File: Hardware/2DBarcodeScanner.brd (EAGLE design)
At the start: 43.2 x 35.6 mm, 53 parts, among them J1 BARCODE_ENGINE_CONN, Q1 600mA/40V, Q2 600mA/40V, U1 3.3V, U5 CH340C

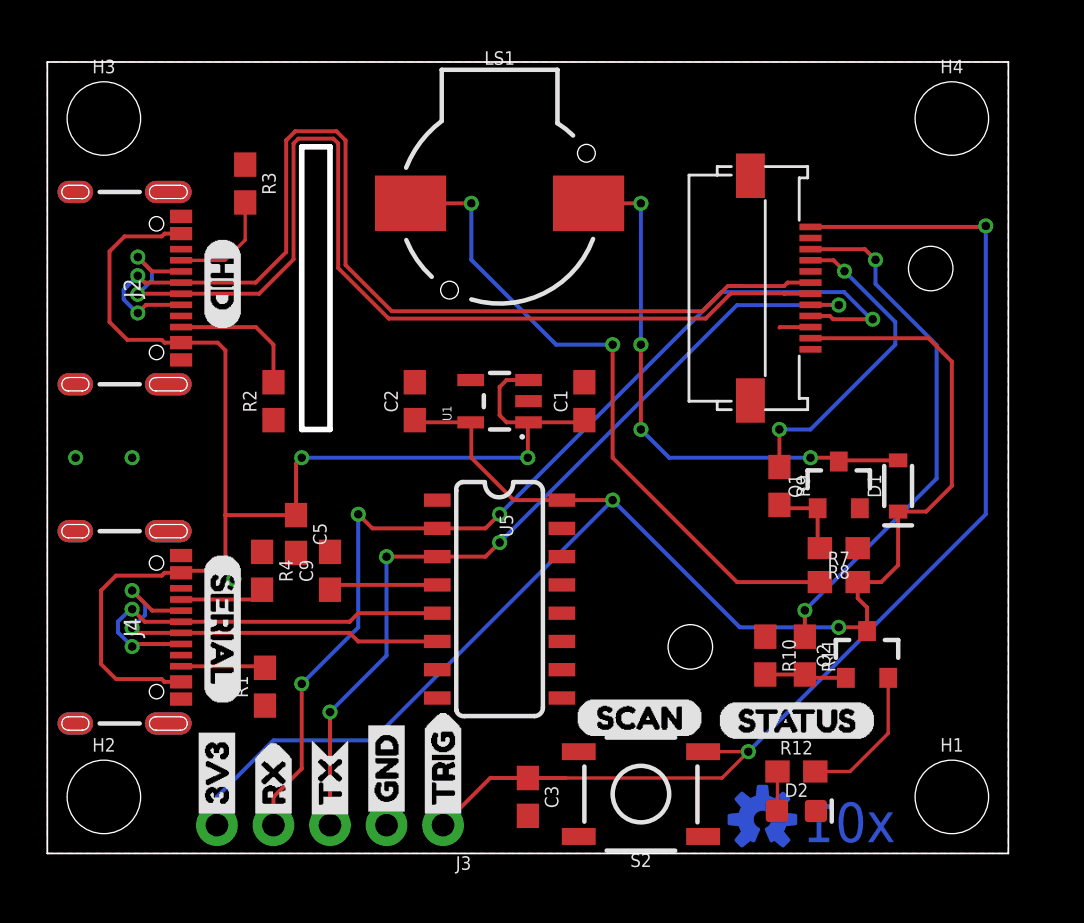
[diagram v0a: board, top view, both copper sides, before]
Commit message: Version x02
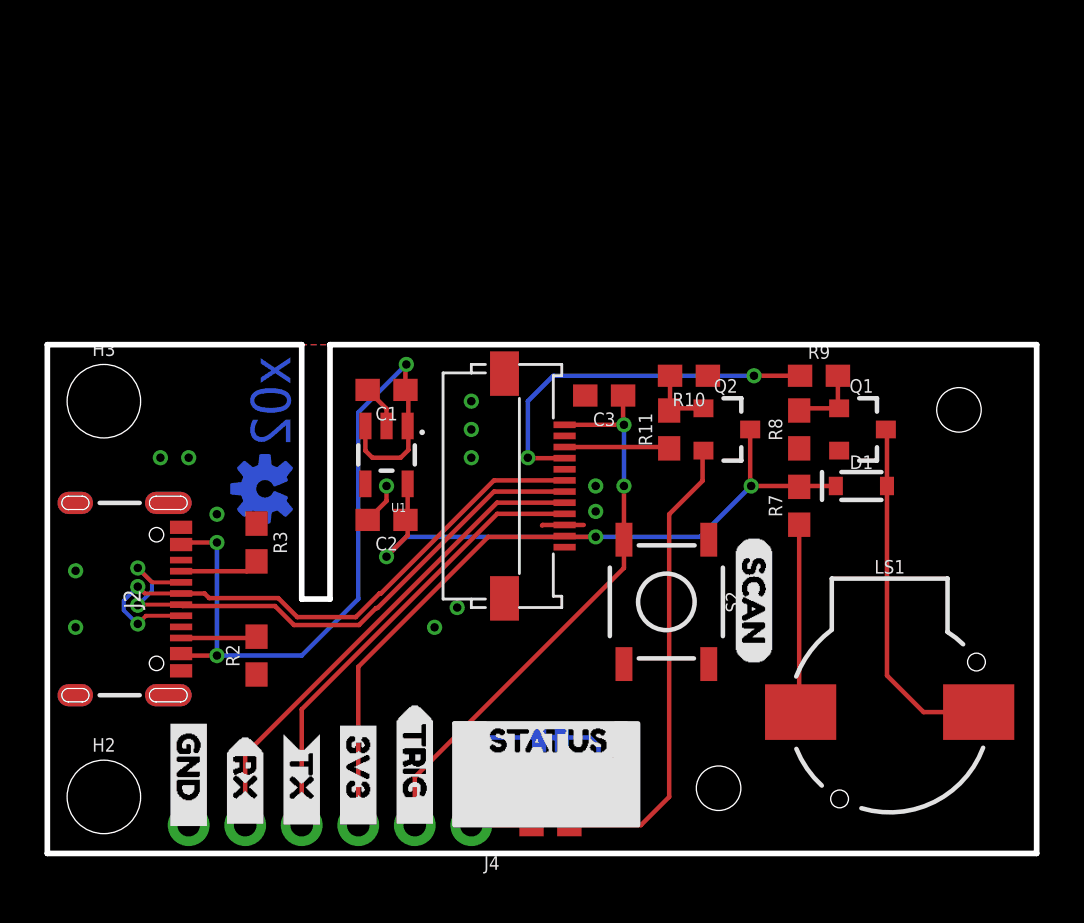
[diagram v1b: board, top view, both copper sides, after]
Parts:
- removed C5: 0.1uF, SparkFun-Capacitors:0603
- removed C9: 10nF, SparkFun-Capacitors:0603
- removed H1, H4: STAND-OFF, SparkFun-Hardware:STAND-OFF
- removed J3: (no value), SparkFun-Connectors:1X05_NO_SILK
- removed R12: 1k, SparkFun-Resistors:0603
- removed R4: 5.1k, SparkFun-Resistors:0603
- removed U$16: (no value), buzzard_labels:HID5
- removed U$19: (no value), buzzard_labels:SERIAL6
- removed U5: CH340C, SparkFun-IC-Comms:SO016
- added JP1: JUMPER-SMT_2_NC_TRACE_SILK, SparkFun-Jumpers:SMT-JUMPER_2_NC_TRACE_SILK
- J4: device SparkFun-Connectors:USB-C-16P -> SparkFun-Connectors:1X06_NO_SILK
- R1: value 5.1k -> 470
- U$10: device buzzard_labels:SERIAL6 -> buzzard_labels (32):TX__2
- U$11: device Labels:3V3-04 -> buzzard_labels (32):TX__2
- U$12: device buzzard_labels:RX0 -> buzzard_labels (32):RX__1
- U$13: device buzzard_labels:TX1 -> buzzard_labels (32):RX__1
- U$14: device Labels:GND-04 -> buzzard_labels (32):GND__0
- U$15: device buzzard_labels (2):TRIG2 -> buzzard_labels (32):GND__0
- U$2: device Labels:GND-04 -> buzzard_labels:STATUS3
- U$3: device Labels:3V3-04 -> buzzard_labels (32):STAT__5
- U$4: device buzzard_labels:RX0 -> buzzard_labels (32):TRIG__4
- U$5: device buzzard_labels:TX1 -> buzzard_labels (32):TRIG__4
- U$6: device buzzard_labels (2):TRIG2 -> buzzard_labels (32):3V3__3
- U$8: device buzzard_labels:STATUS3 -> buzzard_labels (33):LED0
- U$9: device buzzard_labels:HID5 -> buzzard_labels (32):3V3__3
- moved LS1 28.8 mm to (37.8, 6.35)
- moved U$21 26.8 mm to (9.78, 16.4), turned to 270 degrees
- moved U$9 21.4 mm to (14.0, 6.22), turned to 270 degrees
- moved C3 18.4 mm to (25.0, 20.6), turned to 180 degrees
- moved R3 16.1 mm to (9.40, 14.0)
- moved J4 15.5 mm to (19.1, 1.27), turned to 180 degrees
- moved R1 14.3 mm to (22.6, 1.27), turned to 0 degrees
- moved J1 14.2 mm to (23.2, 16.5)
- moved J2 14.0 mm to (6.35, 11.4)
- moved R10 13.0 mm to (28.8, 21.5), turned to 180 degrees
- moved U$3 12.7 mm to (19.1, 6.86), flipped to the bottom, turned to 270 degrees
- moved H3 12.7 mm to (2.54, 20.3)
- moved U$15 12.5 mm to (6.35, 6.35), flipped to the top, turned to 270 degrees
- moved Q2 12.0 mm to (30.5, 19.1), turned to 270 degrees
- moved R11 11.8 mm to (27.9, 19.1), turned to 90 degrees
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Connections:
- removed net CC1: J4.A5, R4.2
- removed net CC2: J4.B5, R1.2
- removed net D+: J4.A6, J4.B6, U5.5
- removed net D-: J4.A7, J4.B7, U5.6
- removed net N$1: C9.1, U5.4
- removed net N$6: D2.A, R12.1
- new net N$8: D2.A, JP1.1
- new net STATUS_OUT: J4.1, JP1.2, R1.1
- net 3.3V: now also J4.3; no longer J3.5, U5.16
- net 5V: no longer C5.1, J4.VBUS1, J4.VBUS2
- net GND: now also J4.6; no longer C5.2, C9.2, J3.2, J4.GND, J4.GND2, R1.1, R4.1, U5.1
- net N$4: now also R1.2; no longer R12.2
- net RXI: now also J4.5; no longer J3.3, U5.3
- net SCAN_TRIGGER: now also J4.2; no longer J3.1
- net SHLD: no longer J4.SHLD1, J4.SHLD2, J4.SHLD3, J4.SHLD4, J4.SHLD5, J4.SHLD6, J4.SHLD7, J4.SHLD8
- net TXO: now also J4.4; no longer J3.4, U5.2
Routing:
- net SCAN_TRIGGER: track 53.1 -> 25.9 mm
- net TXO: track 46.7 -> 20.7 mm, vias 4 -> 0
- net 5V: track 59.7 -> 34.5 mm, vias 2 -> 3
- net 3.3V: track 72.0 -> 48.1 mm, vias 2 -> 3
- net N$3: track 29.9 -> 8.45 mm, vias 2 -> 0
- net USB_N: track 47.7 -> 26.5 mm
- net USB_P: track 47.6 -> 26.6 mm
- net STATUS_LED: track 23.6 -> 4.72 mm, vias 2 -> 0
- net D-: track 18.7 -> 0.00 mm, vias 2 -> 0
- net D+: track 18.6 -> 0.00 mm, vias 2 -> 0
- net RXI: track 39.4 -> 22.2 mm, vias 4 -> 0
- net N$4: track 6.62 -> 21.2 mm
- net STATUS_OUT: track 0.00 -> 9.39 mm
- net N$2: track 24.7 -> 15.9 mm, vias 4 -> 0
- net N$1: track 4.91 -> 0.00 mm
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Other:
- board size 43.2 x 35.6 mm -> 44.5 x 22.9 mm
- board text added: "x02"
- board text removed: "x01"
